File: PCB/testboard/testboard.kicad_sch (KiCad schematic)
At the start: 11 parts, among them Q1 IRF3205, Q2 IRF3205, U6 IR2104

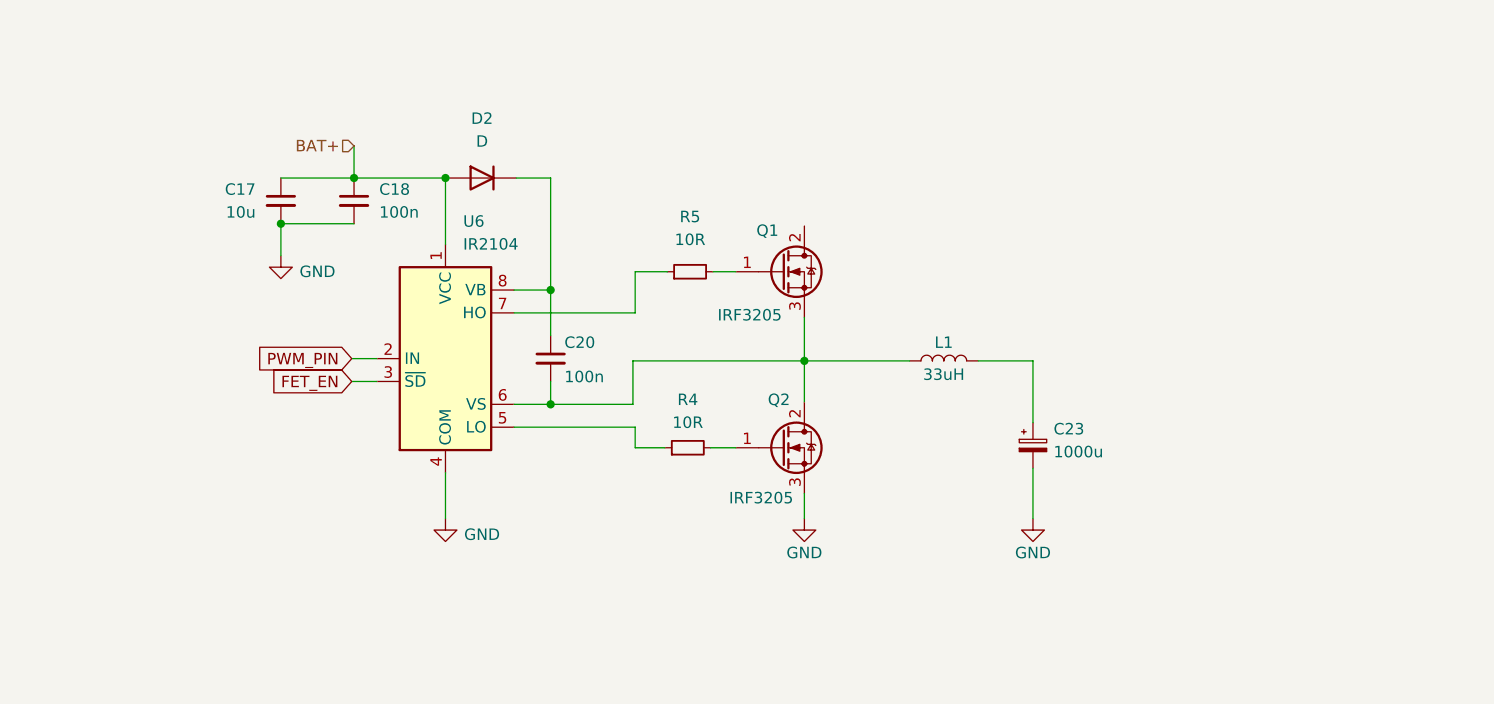
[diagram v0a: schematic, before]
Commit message: update test board and docs
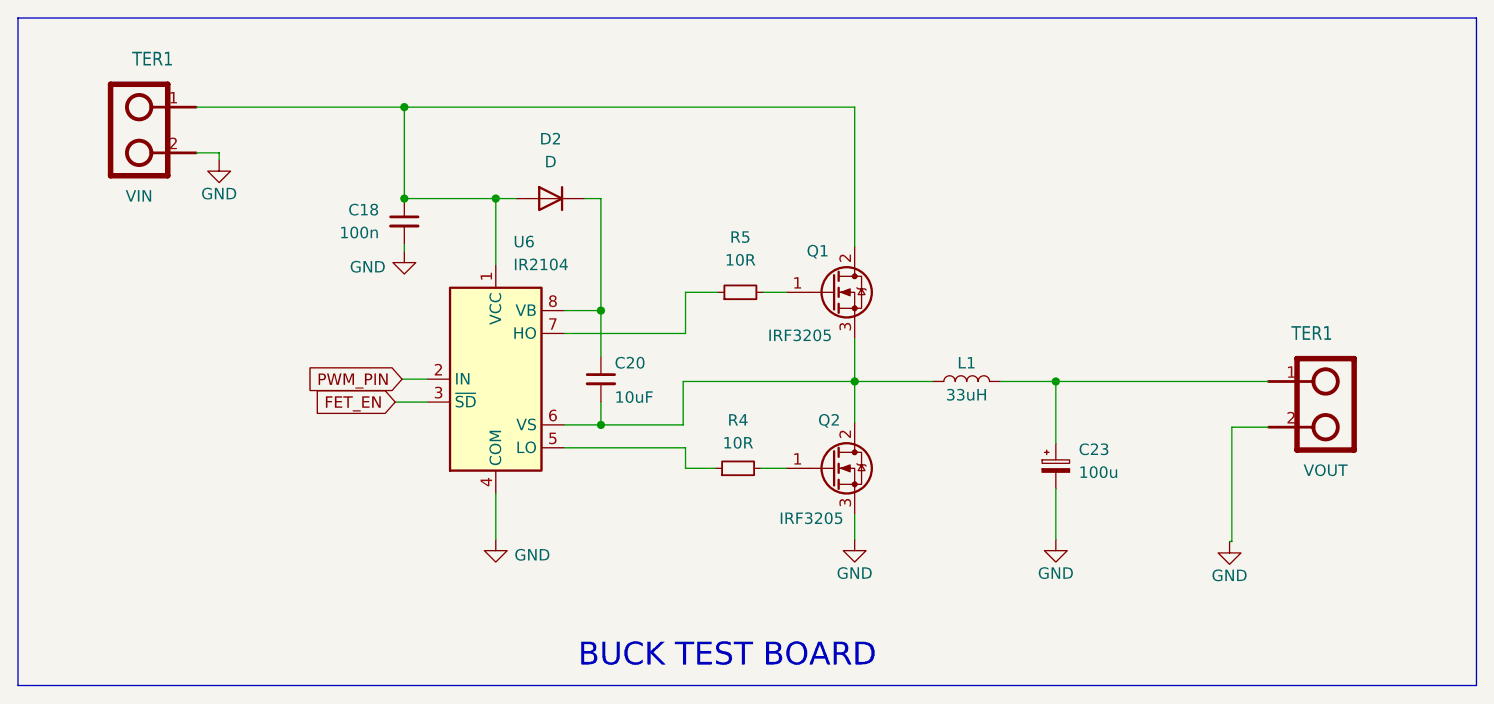
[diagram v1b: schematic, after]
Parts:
- removed C17: 10u, symbol Device:C_Small
- added TER1: VIN, Project232:DOMI-2, symbol Project232-eagle-import:DOMINO-2
- added TER1: VOUT, Project232:DOMI-2, symbol Project232-eagle-import:DOMINO-2
- C20: value 100n -> 10uF
- C23: value 1000u -> 100u
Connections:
- net BAT+ is gone; now on an unnamed net: C18.1, D2.2 (A), U6.1 (VCC)
- net GND: now also TER1.2, TER1.2
- net at Q1.2 (D): now also TER1.1
- net at C23.1, L1.2: now also TER1.1
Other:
- note added: "BUCK TEST BOARD"

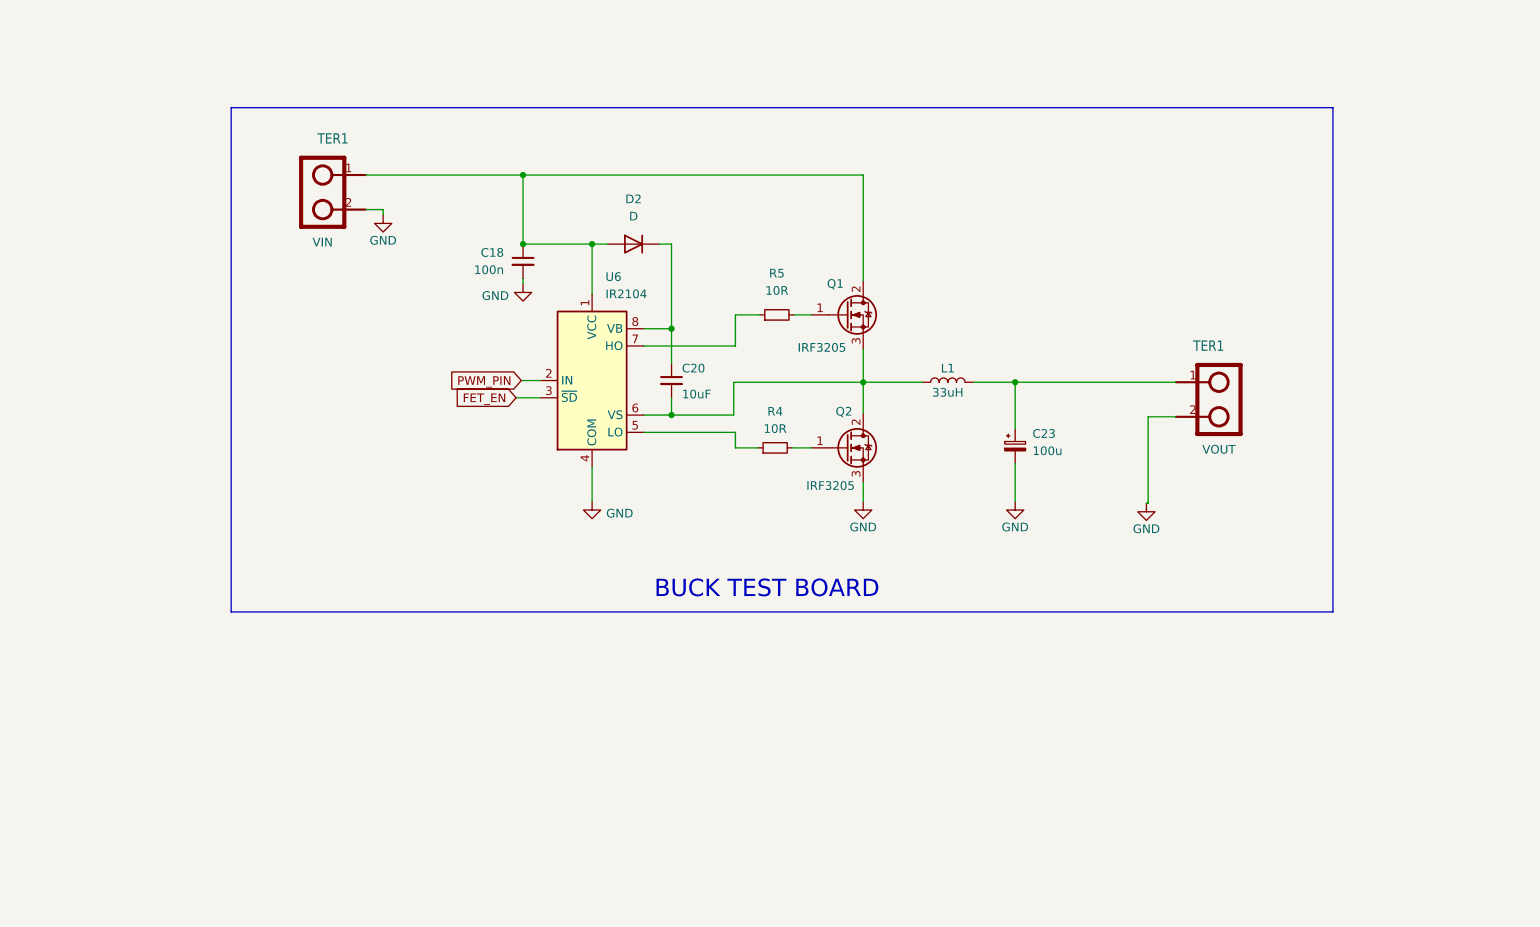
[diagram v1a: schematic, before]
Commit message: Update PCB
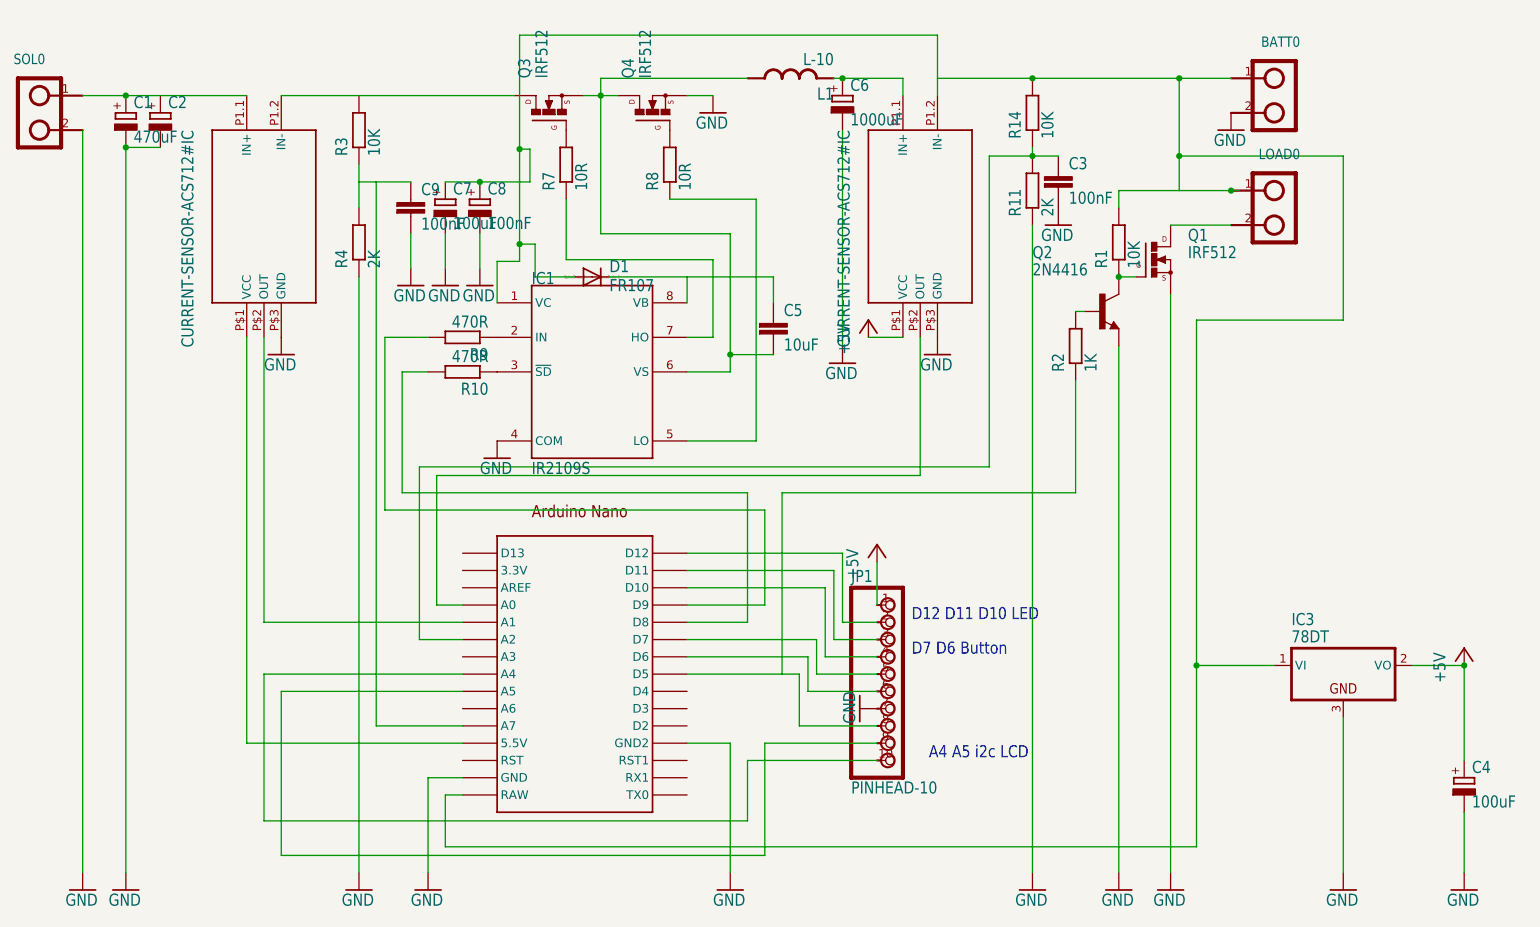
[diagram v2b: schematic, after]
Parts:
- removed C18: 100n, symbol Device:C_Small
- removed C20: 10uF, symbol Device:C_Small
- removed C23: 100u, symbol Device:C_Polarized_Small
- removed D2: D, symbol Device:D
- removed L1: 33uH, symbol Device:L
- removed Q1, Q2: IRF3205, Package_TO_SOT_THT:TO-220-3_Vertical, symbol Transistor_FET:IRF3205
- removed R4, R5: 10R, symbol Device:R_Small
- removed TER1: VIN, Project232:DOMI-2, symbol Project232-eagle-import:DOMINO-2
- removed TER1: VOUT, Project232:DOMI-2, symbol Project232-eagle-import:DOMINO-2
- removed U6: IR2104, symbol Driver_FET:IR2104
- added .0, U$3: CURRENT-SENSOR-ACS712#IC, testboard:CURRENT-SENSOR-ACS712#IC, symbol testboard-eagle-import:CURRENT-SENSOR-ACS712#IC
- added BATT0, LOAD0, SOL0: DOMINO-2, testboard:DOMI-2, symbol testboard-eagle-import:DOMINO-2
- added C1: 470uF, testboard:E5-13, symbol testboard-eagle-import:CPOL-EUE5-13
- added C2: CPOL-EUE5-13, testboard:E5-13, symbol testboard-eagle-import:CPOL-EUE5-13
- added C3, C9: 100nF, testboard:C1206, symbol testboard-eagle-import:C-EUC1206
- added C4, C7: 100uF, testboard:SMC_D, symbol testboard-eagle-import:rcl_CPOL-EUSMCD
- added C5: 10uF, testboard:C1812, symbol testboard-eagle-import:C-EUC1812
- added C6: 1000uF, testboard:E5-13, symbol testboard-eagle-import:CPOL-EUE5-13
- added C8: 100nF, testboard:SMC_D, symbol testboard-eagle-import:rcl_CPOL-EUSMCD
- added D1: FR107, testboard:SMB, symbol testboard-eagle-import:DIODE-SMB
- added IC1: IR2109S, testboard:SO08, symbol testboard-eagle-import:IR2109S
- added IC3: 78DT, testboard:TO252, symbol testboard-eagle-import:78DT
- added JP1: PINHEAD-10, testboard:PINHEAD-10, symbol testboard-eagle-import:PINHEAD-10
- added L1: L-10, testboard:L-10, symbol testboard-eagle-import:L-10
- added Q1, Q3: IRF512, testboard:TO220BV, symbol testboard-eagle-import:IRF512
- added Q2: 2N4416, testboard:TO92, symbol testboard-eagle-import:2N4416
- added Q4: IRF512, testboard:TO220BV, symbol testboard-eagle-import:lbr_IRF512
- added R1, R14, R3: 10K, testboard:R1206, symbol testboard-eagle-import:R-EU_R1206
- added R10, R9: 470R, testboard:R1206, symbol testboard-eagle-import:R-EU_R1206
- added R11, R4: 2K, testboard:R1206, symbol testboard-eagle-import:R-EU_R1206
- added R2: 1K, testboard:R1206, symbol testboard-eagle-import:R-EU_R1206
- added R7, R8: 10R, testboard:R1206, symbol testboard-eagle-import:R-EU_R1206
- added U$1: NANO, testboard:NANO, symbol testboard-eagle-import:NANO
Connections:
- net GND: now also .0.P$3 (GND), BATT0.2, C1.-, C2.-, C3.2, C4.-, C6.-, C7.-, C8.-, C9.2, IC1.4 (COM), IC3.3 (GND), JP1.7, Q1.S, Q2.3 (E), Q4.S, R11.1, R4.1, SOL0.2, U$1.GND, U$1.GND1 (GND2), U$3.P$3 (GND)
- new net: C3.1, R11.2, R14.1, U$1.A2
- new net: BATT0.1, C7.+, C8.+, D1.A, IC1.1 (VC), IC3.1 (VI), LOAD0.1, R1.2, R14.2, U$1.RAW, U$3.P1.2 (IN-)
- new net: JP1.8, R2.1, U$1.D5
- new net: Q2.2 (B), R2.2
- new net: C5.1, D1.C, IC1.8 (VB)
- new net: LOAD0.2, Q1.D
- new net: Q1.G, Q2.1 (C), R1.1
- new net: C5.2, IC1.6 (VS), L1.1, Q3.S, Q4.D
- new net: Q4.G, R8.2
- new net: IC1.5 (LO), R8.1
- new net: C6.+, L1.2, U$3.P1.1 (IN+)
- new net: C9.1, R3.1, R4.2, U$1.A7
- new net: JP1.10, U$1.A4
- new net: JP1.2, U$1.D12
- new net: JP1.3, U$1.D11
- new net: JP1.4, U$1.D10
- new net: JP1.5, U$1.D7
- new net: JP1.6, U$1.D6
- new net: JP1.9, U$1.A5
- new net: .0.P$1 (VCC), U$1.5V (5.5V)
- new net: .0.P$2 (OUT), U$1.A1
- new net: .0.P1.1 (IN+), C1.+, C2.+, SOL0.1
- new net: .0.P1.2 (IN-), Q3.D, R3.2
- new net: U$1.A0, U$3.P$2 (OUT)
- new net: R10.2, U$1.D8
- new net: R9.2, U$1.D9
- new net: IC1.3 (~{SD}), R10.1
- new net: IC1.2 (IN), R9.1
- new net: IC1.7 (HO), R7.1
- new net: Q3.G, R7.2
- new net +5V: C4.+, IC3.2 (VO), JP1.1, U$3.P$1 (VCC)
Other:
- note added: "A4 A5 i2c LCD"
- note added: "D12 D11 D10 LED"
- note added: "D7 D6 Button"
- note removed: "BUCK TEST BOARD"
